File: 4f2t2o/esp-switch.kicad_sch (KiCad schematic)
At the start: 62 parts, among them J2 Screw_Terminal_01x04, J3 Screw_Terminal_01x04, J4 Conn_02x04_Odd_Even, J5 Screw_Terminal_01x04, J7 Screw_Terminal_01x04, Q1 TSM2302CX, Q2 TSM2302CX, Q3 TSM2302CX, Q4 TSM2302CX, Q5 BT138-600, Q6 BT138-600, U1 VOT-8024, U2 ESP-12E, U3 tlp785gb, U4 tlp785gb, U5 TPS54202DDC, U6 VOT-8024

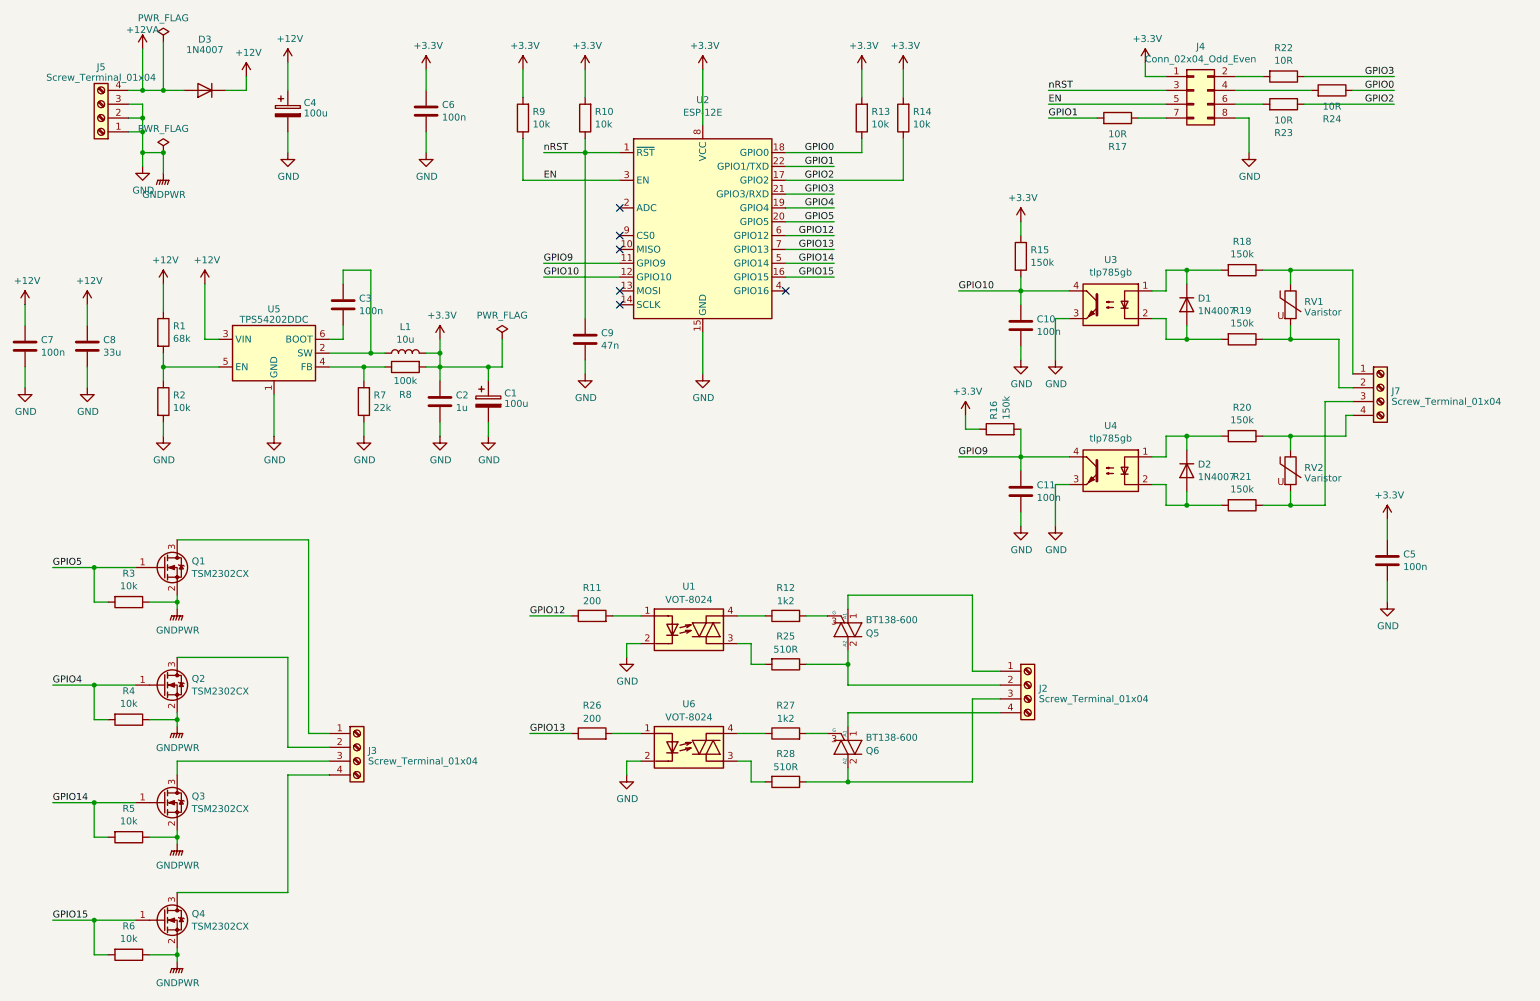
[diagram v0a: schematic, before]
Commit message: v0.1 for 8f2o and 4f2t2o
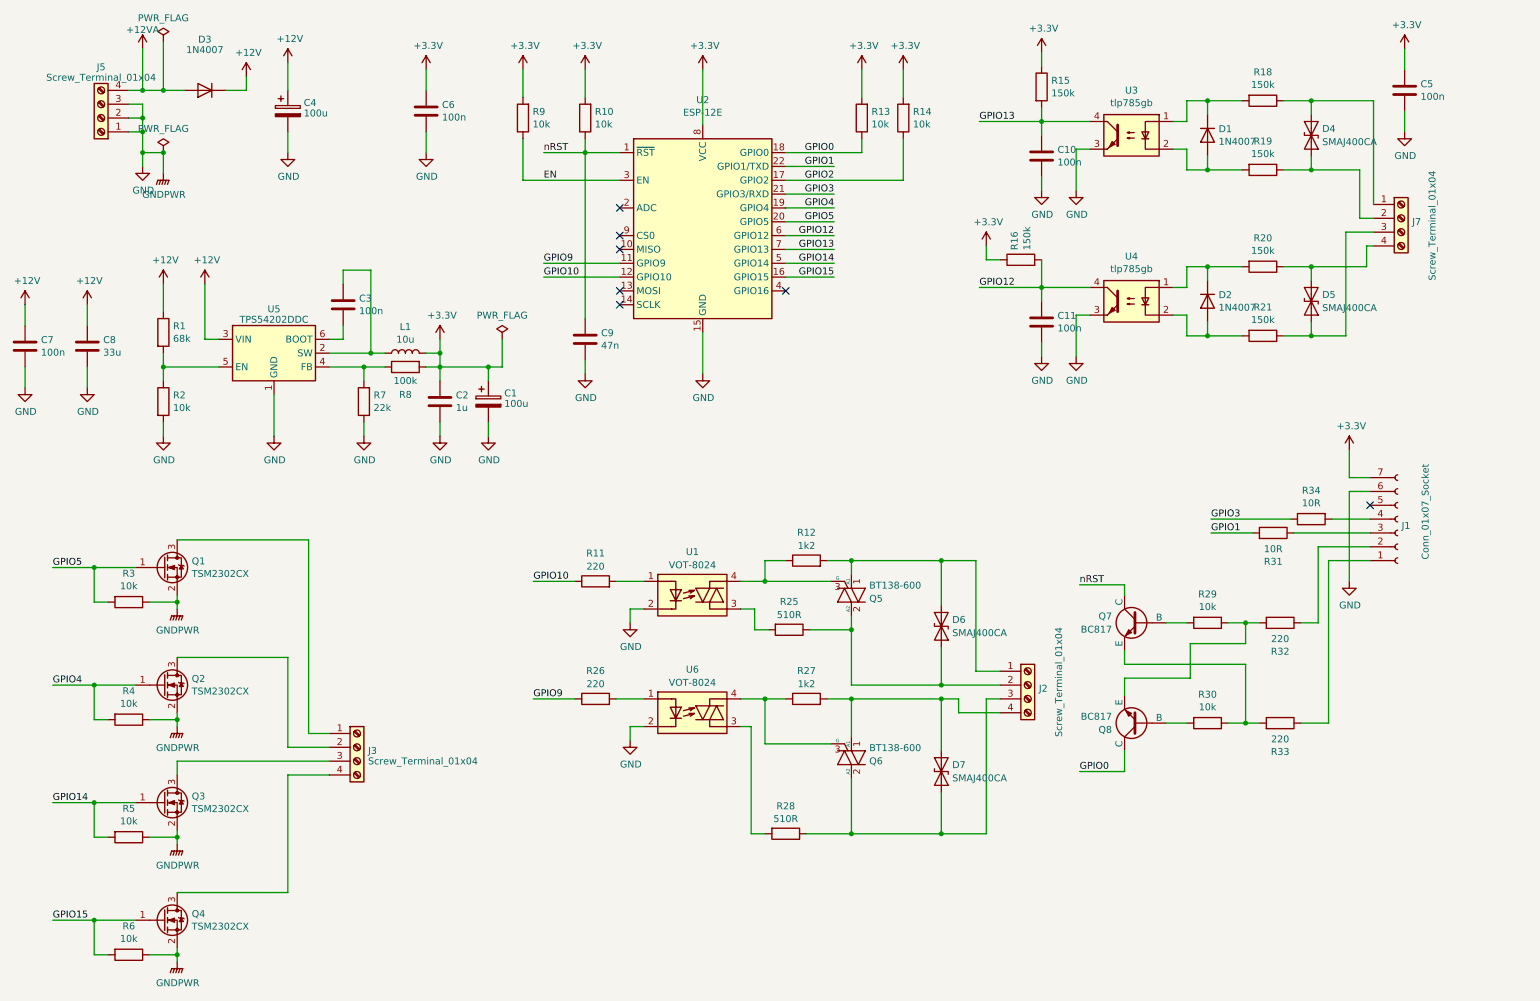
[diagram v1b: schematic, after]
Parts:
- removed J4: Conn_02x04_Odd_Even, Connector_PinHeader_2.54mm:PinHeader_2x04_P2.54mm_Vertical, symbol Connector_Generic:Conn_02x04_Odd_Even
- removed R17, R22, R23, R24: 10R, Resistor_SMD:R_0805_2012Metric_Pad1.20x1.40mm_HandSolder, symbol Device:R
- removed RV1, RV2: Varistor, Varistor:RV_Disc_D7mm_W5.7mm_P5mm, symbol Device:Varistor
- added D4, D5, D6, D7: SMAJ400CA, Diode_SMD:D_SMA, symbol Diode:SMAJ400CA
- added J1: Conn_01x07_Socket, Connector_PinSocket_2.54mm:PinSocket_1x07_P2.54mm_Horizontal, symbol Connector:Conn_01x07_Socket
- added Q7, Q8: BC817, Package_TO_SOT_SMD:SOT-23_Handsoldering, symbol Simulation_SPICE:NPN
- added R29, R30: 10k, Resistor_SMD:R_0805_2012Metric_Pad1.20x1.40mm_HandSolder, symbol Device:R
- added R31, R34: 10R, Resistor_SMD:R_0805_2012Metric_Pad1.20x1.40mm_HandSolder, symbol Device:R
- added R32, R33: 220, Resistor_SMD:R_0805_2012Metric_Pad1.20x1.40mm_HandSolder, symbol Device:R
- Q1, Q2, Q3, Q4: Farnell (none) -> 3121715
- Q5, Q6: footprint Package_TO_SOT_THT:TO-220-3_Vertical -> esp-switch:TO-220-3_Vertical_offset
- R11, R26: value 200 -> 220
- U1, U6: Farnell (none) -> 3778033
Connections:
- net +3V3: now also J1.7 (Pin_7)
- net GND: now also J1.6 (Pin_6)
- net GPIO0: now also Q8.1 (C)
- net GPIO1: now also R31.2
- net GPIO10: now also R11.1; no longer C10.1, R15.2, U3.4
- net GPIO12: now also C11.1, R16.2, U4.4; no longer R11.1
- net GPIO13: now also C10.1, R15.2, U3.4; no longer R26.1
- net GPIO3: now also R34.1
- net GPIO9: now also R26.1; no longer C11.1, R16.2, U4.4
- net nRST: now also Q7.1 (C)
- net at J7.1 (Pin_1), R18.1: now also D4.2 (A2)
- net at J7.2 (Pin_2), R19.1: now also D4.1 (A1)
- net at J7.4 (Pin_4), R20.1: now also D5.2 (A2)
- net at J7.3 (Pin_3), R21.1: now also D5.1 (A1)
- net at R27.1, U6.4 (R): now also Q6.3 (G)
- net at R27.2: now also J2.4 (Pin_4), Q6.1 (A1), D7.2 (A2); no longer Q6.3 (G)
- net at J2.1 (Pin_1), Q5.1 (A1): now also R12.2, D6.2 (A2)
- net at J2.2 (Pin_2), Q5.2 (A2), R25.1: now also D6.1 (A1)
- net at Q5.3 (G): now also R12.1, U1.4 (R); no longer R12.2
- net at J2.3 (Pin_3), Q6.2 (A2), R28.1: now also D7.1 (A1)
- new net: Q8.3 (E), R29.1, R32.2
- new net: Q7.2 (B), R29.2
- new net: J1.1 (Pin_1), R33.1
- new net: J1.2 (Pin_2), R32.1
- new net: J1.3 (Pin_3), R31.1
- new net: J1.4 (Pin_4), R34.2
- new net: Q8.2 (B), R30.2
- new net: Q7.3 (E), R30.1, R33.2
- no-connect marks 6 -> 7
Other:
- moved on the sheet: C10, C11, C5, D1, D2, J7, Q5, Q6, R11, R12, R15, R16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
